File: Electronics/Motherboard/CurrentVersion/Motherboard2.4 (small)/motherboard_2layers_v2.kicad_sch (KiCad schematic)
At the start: 87 parts, among them J1 Conn_02x10_Odd_Even, J2 SSD1306, J3 USB_C_Receptacle_USB2.0_16P, J4 Micro_SD_Card_Det2, J5 Encoder, Q1 FDMS86202, Q2 FDMS86202, Q3 AO3400A, Q4 AO3400A, Q5 AO3400A, U1 TMC2209_SilentStepStick, U2 TMC2209_SilentStepStick, U3 LY1576HVS-5, U4 TMC2209_SilentStepStick, U5 TMC2209_SilentStepStick, U6 STZ12F405RGTx, U7 AMS1117-3.3, U8 AW9523B, U9 USBLC6-2SC6

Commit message: tinny pcb
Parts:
- C23, C24: footprint Capacitor_SMD:C_1206_3216Metric -> Capacitor_SMD:C_0603_1608Metric
- D1: footprint Diode_THT:D_DO-201AD_P15.24mm_Horizontal -> Diode_SMD:D_SOD-123; Part # 1N5822 -> C2972823
- R10, R9: footprint Resistor_SMD:R_0805_2012Metric -> Resistor_SMD:R_0402_1005Metric
- R11, R2, R3: footprint Resistor_SMD:R_1206_3216Metric -> Resistor_SMD:R_0603_1608Metric
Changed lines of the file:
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@@
 			)
 		)
-		(property "Footprint" "Resistor_SMD:R_0805_2012Metric"
+		(property "Footprint" "Resistor_SMD:R_0402_1005Metric"
 			(at 138.43 241.808 90)
 			(effects
@@
 			)
 		)
-		(property "Footprint" "Resistor_SMD:R_1206_3216Metric"
+		(property "Footprint" "Resistor_SMD:R_0603_1608Metric"
 			(at 137.922 132.08 90)
 			(effects
@@
 			)
 		)
-		(property "Footprint" "Diode_THT:D_DO-201AD_P15.24mm_Horizontal"
+		(property "Footprint" "Diode_SMD:D_SOD-123"
 			(at 199.39 101.6 0)
 			(effects
@@
 			)
 		)
-		(property "Part #" "1N5822"
+		(property "Part #" "C2972823"
 			(at 199.39 101.6 90)
 			(effects
@@
 			)
 		)
-		(property "Footprint" "Resistor_SMD:R_0805_2012Metric"
+		(property "Footprint" "Resistor_SMD:R_0402_1005Metric"
 			(at 138.43 249.428 90)
 			(effects
@@
 			)
 		)
-		(property "Footprint" "Resistor_SMD:R_1206_3216Metric"
+		(property "Footprint" "Resistor_SMD:R_0603_1608Metric"
 			(at 122.682 134.62 90)
 			(effects
@@
 			)
 		)
-		(property "Footprint" "Capacitor_SMD:C_1206_3216Metric"
+		(property "Footprint" "Capacitor_SMD:C_0603_1608Metric"
 			(at 43.4848 157.48 0)
 			(effects
@@
 			)
 		)
-		(property "Footprint" "Capacitor_SMD:C_1206_3216Metric"
+		(property "Footprint" "Capacitor_SMD:C_0603_1608Metric"
 			(at 30.7848 157.48 0)
 			(effects
@@
 			)
 		)
-		(property "Footprint" "Resistor_SMD:R_1206_3216Metric"
+		(property "Footprint" "Resistor_SMD:R_0603_1608Metric"
 			(at 29.972 274.32 90)
 			(effects

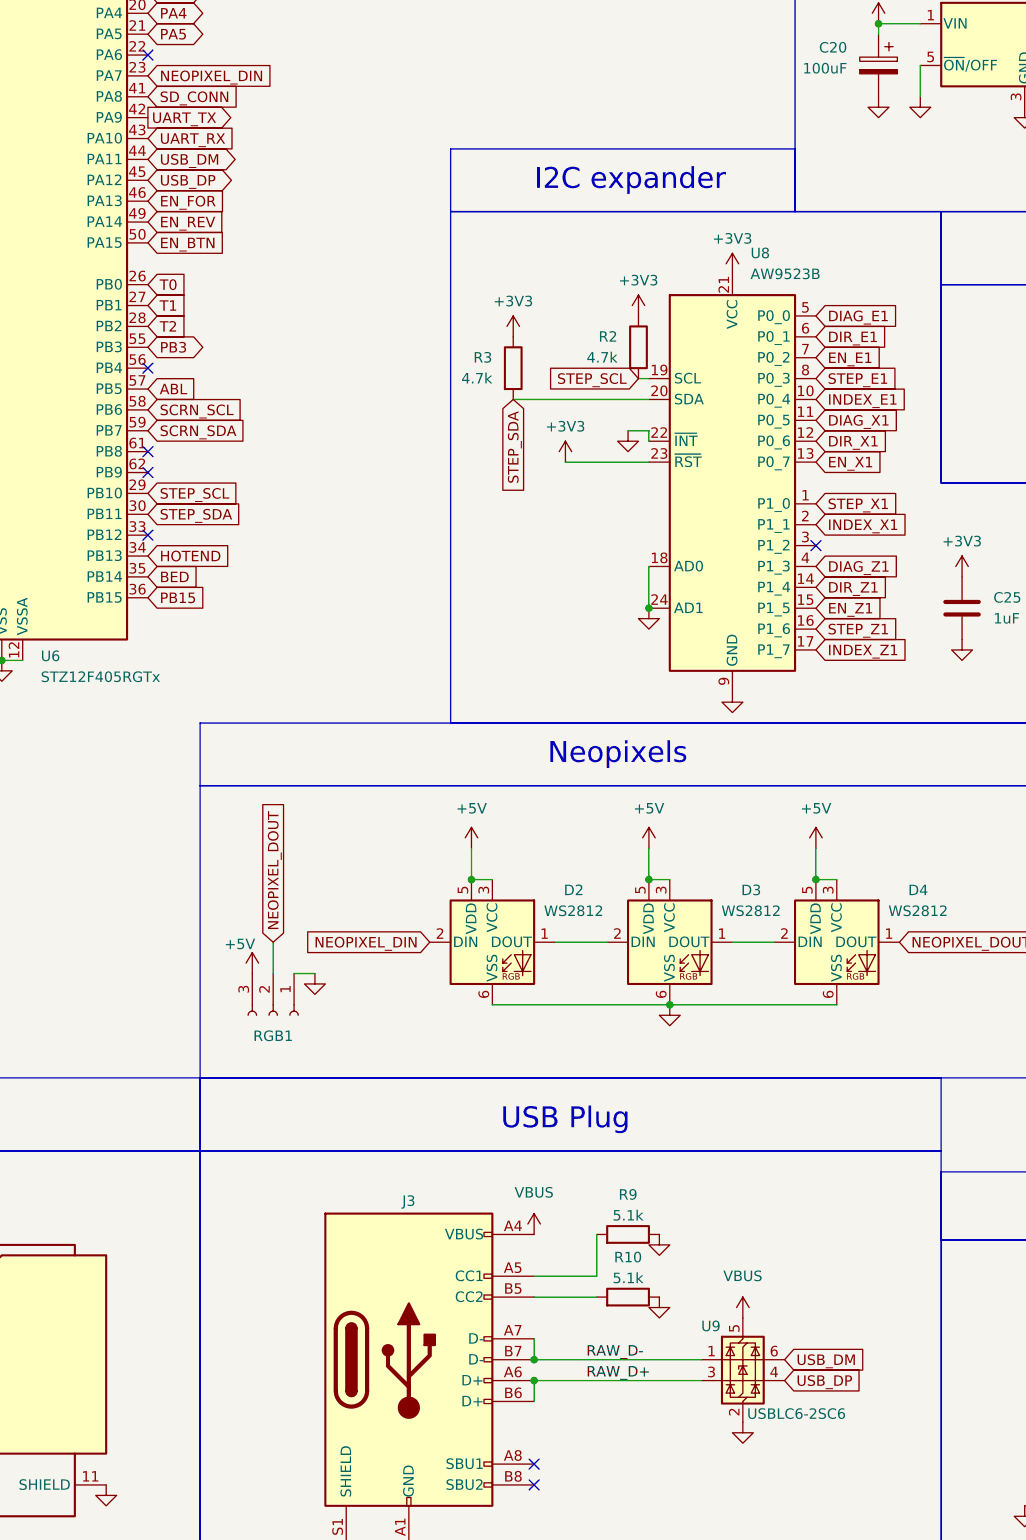
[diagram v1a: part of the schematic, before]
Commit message: Started routing
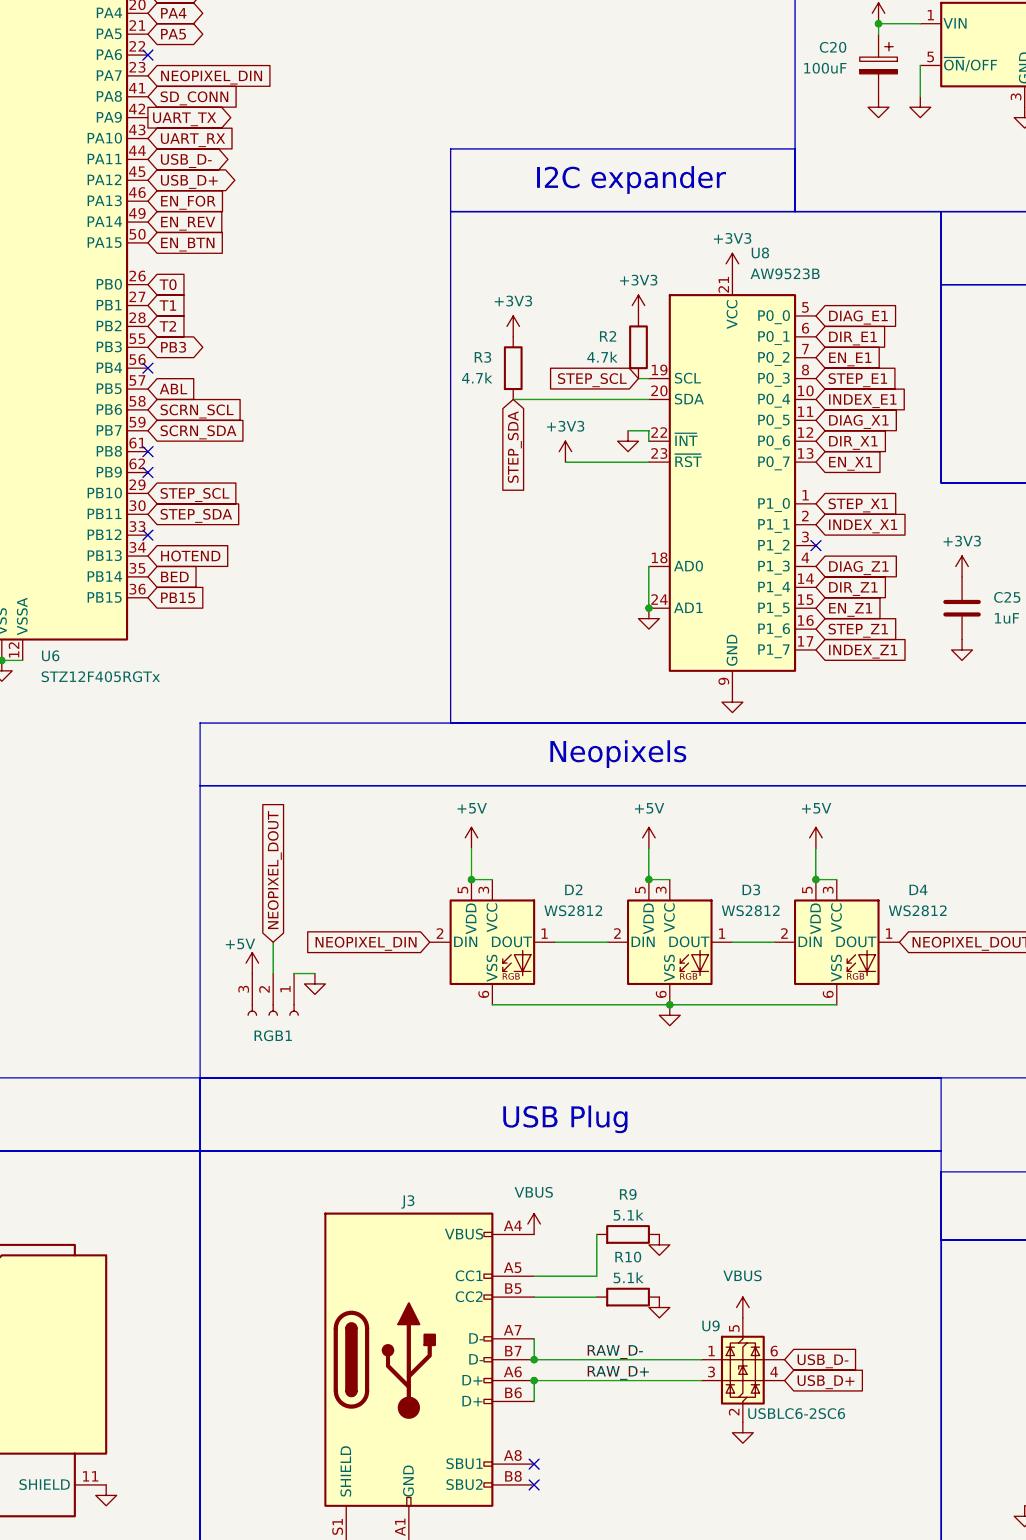
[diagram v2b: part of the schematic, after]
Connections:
- net USB_DM renamed USB_D-
- net USB_DP renamed USB_D+
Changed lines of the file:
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@@
 		)
 	)
-	(global_label "USB_DM"
+	(global_label "USB_D-"
 		(shape bidirectional)
 		(at 80.01 109.22 0)
@@
 		)
 	)
-	(global_label "USB_DM"
+	(global_label "USB_D-"
 		(shape input)
 		(at 157.48 255.27 0)
@@
 		)
 	)
-	(global_label "USB_DP"
+	(global_label "USB_D+"
 		(shape bidirectional)
 		(at 80.01 111.76 0)
@@
 		)
 	)
-	(global_label "USB_DP"
+	(global_label "USB_D+"
 		(shape input)
 		(at 157.48 257.81 0)

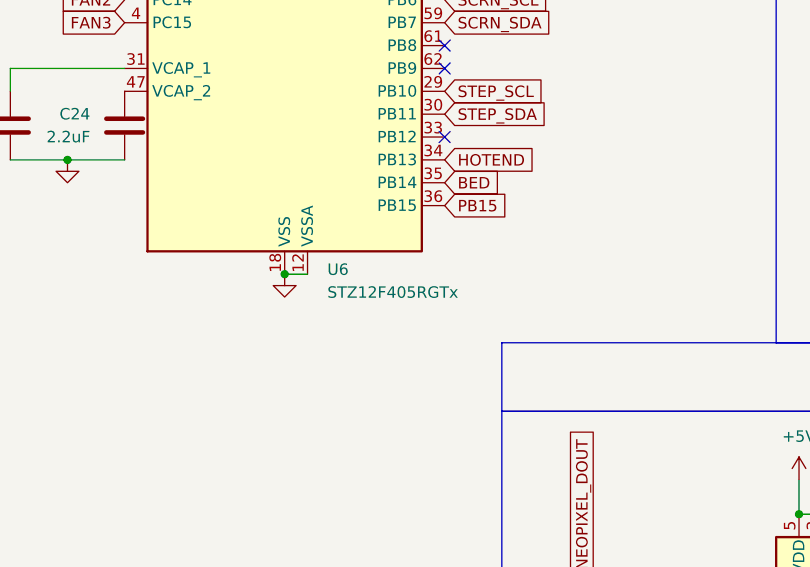
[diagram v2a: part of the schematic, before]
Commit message: Fixed a typo that's been there for idk how long
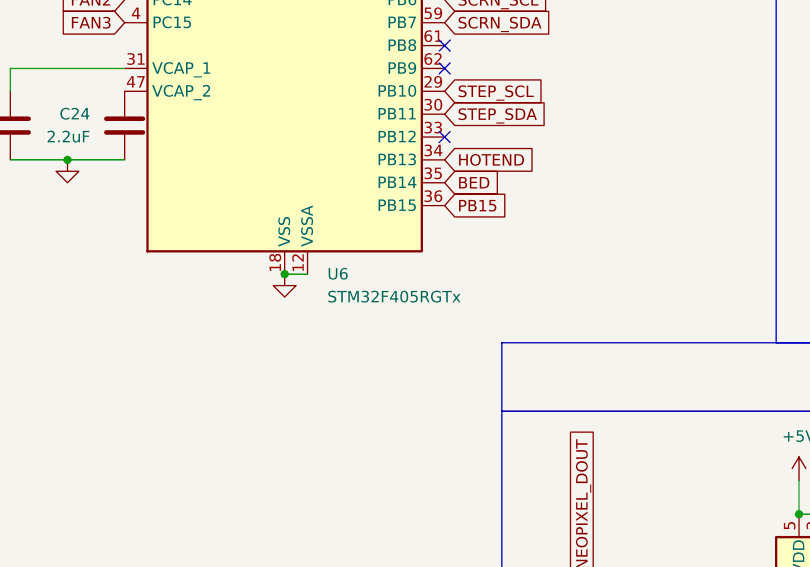
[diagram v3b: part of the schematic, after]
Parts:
- U6: value STZ12F405RGTx -> STM32F405RGTx
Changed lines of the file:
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@@
 		(fields_autoplaced yes)
 		(property "Reference" "U6"
-			(at 66.9641 169.672 0)
+			(at 66.9641 170.18 0)
 			(effects
 				(font
@@
 			)
 		)
-		(property "Value" "STZ12F405RGTx"
-			(at 66.9641 172.212 0)
+		(property "Value" "STM32F405RGTx"
+			(at 66.9641 172.72 0)
 			(effects
 				(font
